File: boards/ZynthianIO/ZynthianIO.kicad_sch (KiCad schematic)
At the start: 27 parts, among them J1 Btn-1, J1 Raspberry_Pi_2_3, J10 Ctrl-2, J11 Display, J3 Btn-2, J7 Ctrl-3, J8 Ctrl-4, J9 Ctrl-1, U1 MCP23017_SP, U2 6N138, U3 74LS14

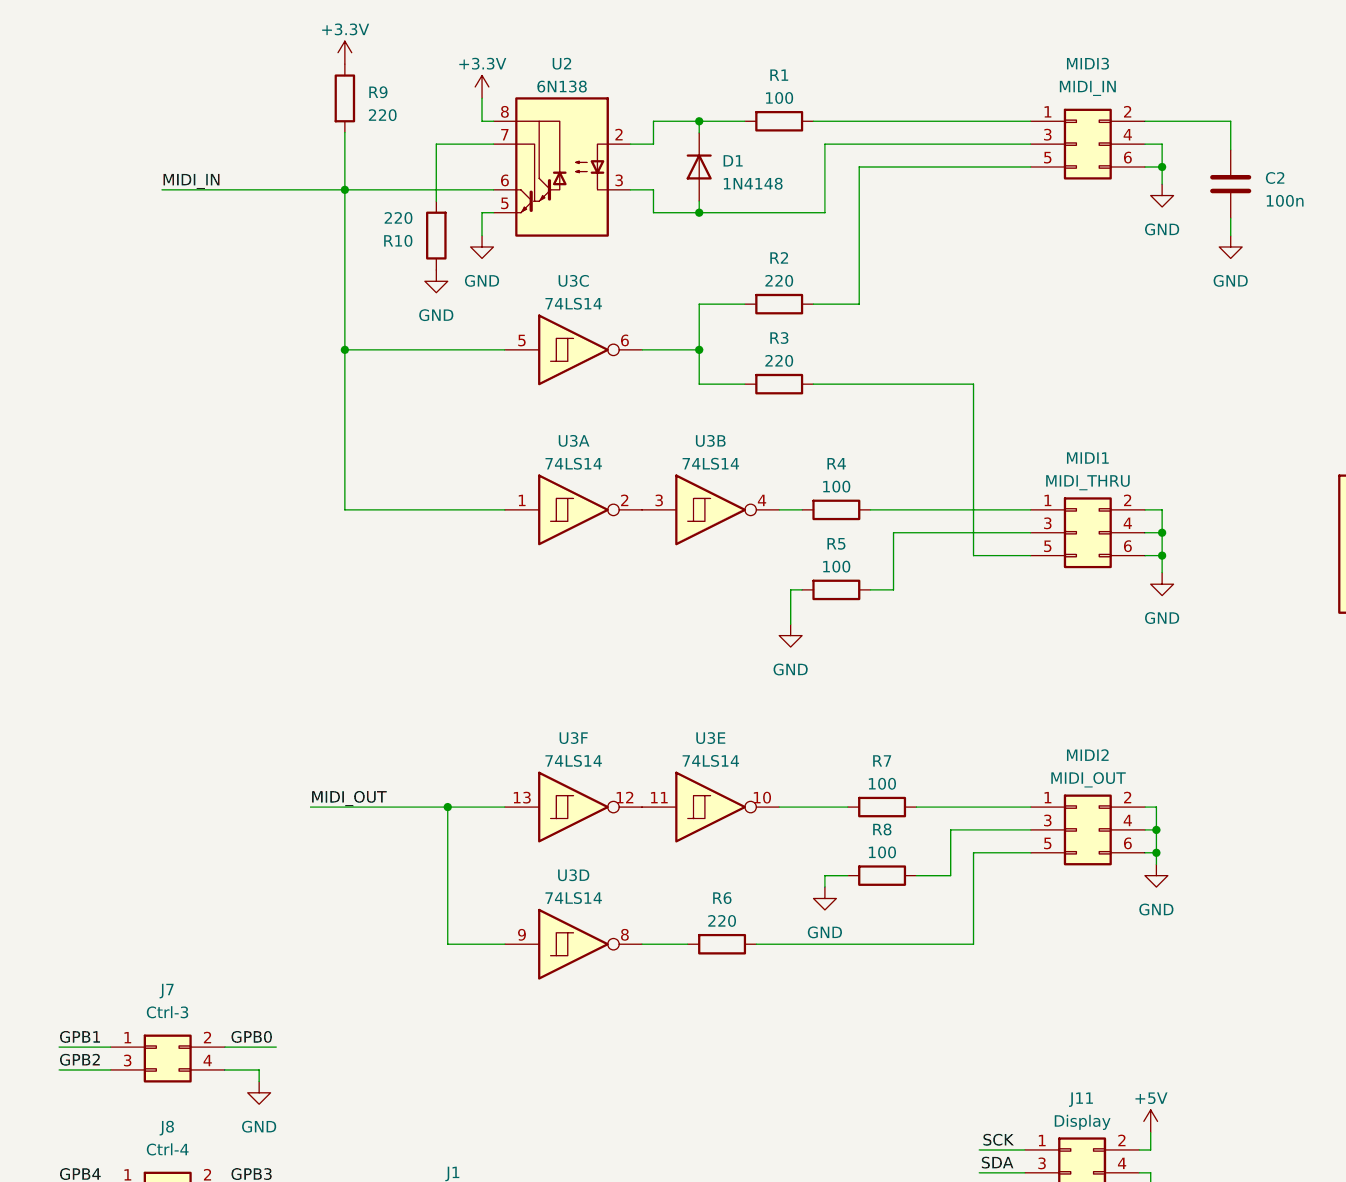
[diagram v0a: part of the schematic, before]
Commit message: Fixed MIDI interfaces
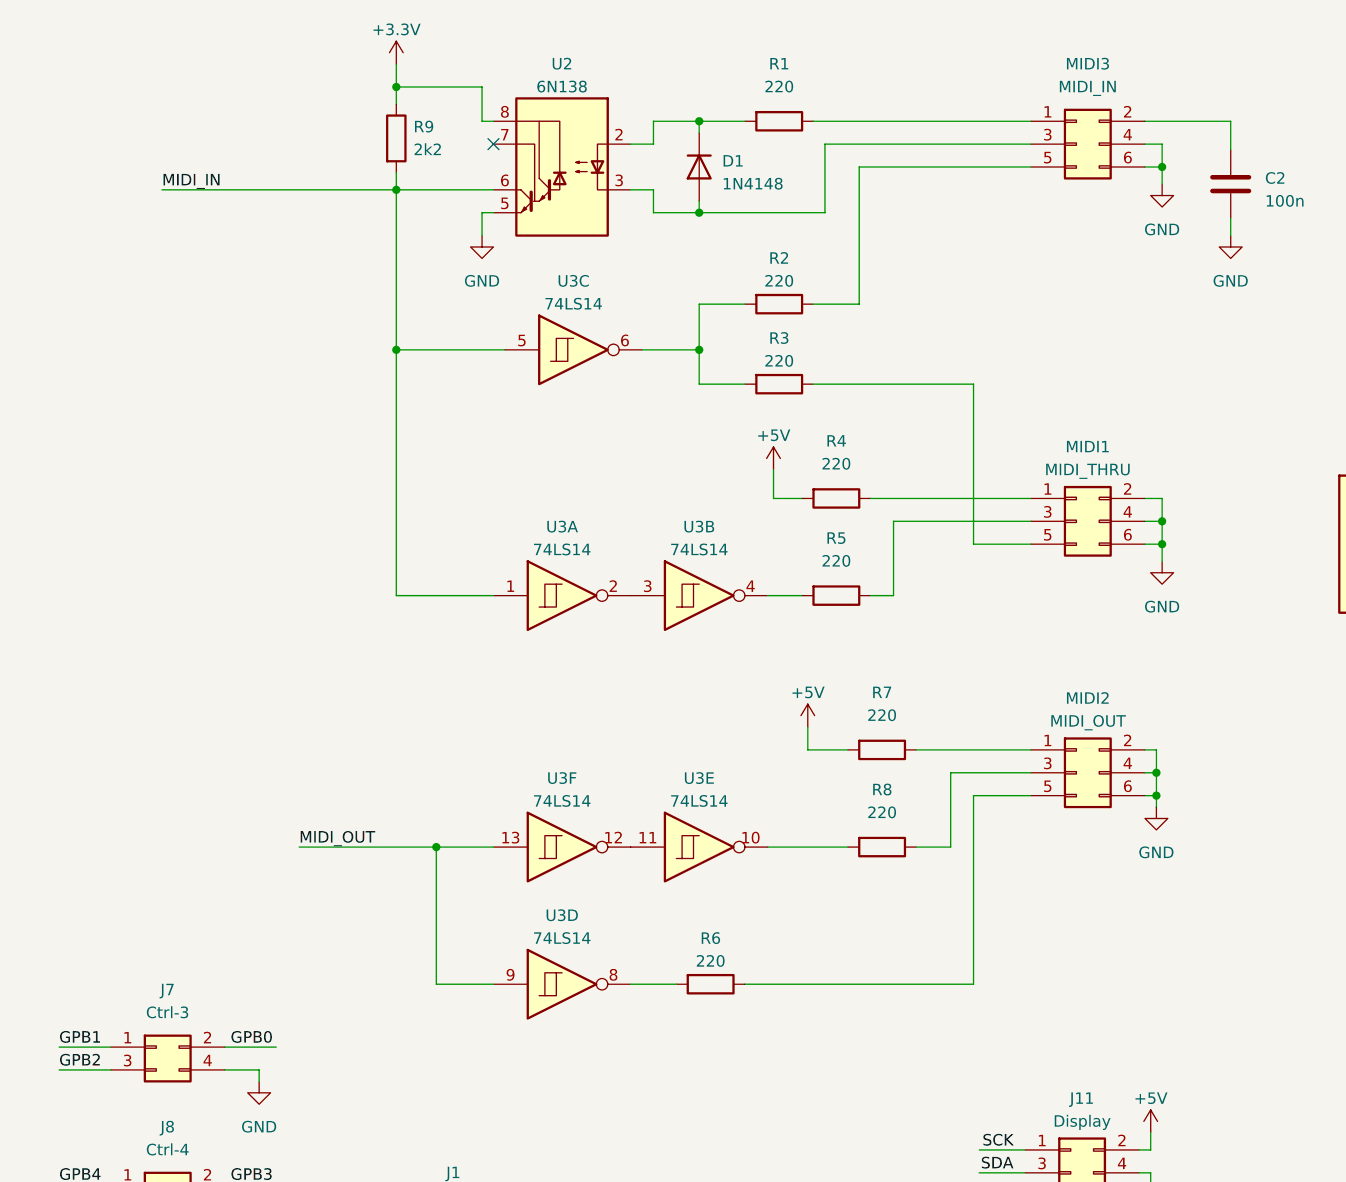
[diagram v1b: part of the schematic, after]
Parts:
- removed R10: 220, Resistor_THT:R_Axial_DIN0207_L6.3mm_D2.5mm_P7.62mm_Horizontal, symbol Device:R
- D1: footprint Diode_THT:D_DO-34_SOD68_P7.62mm_Horizontal -> Diode_THT:D_DO-35_SOD27_P7.62mm_Horizontal
- R1, R4, R5, R7, R8: value 100 -> 220
- R9: value 220 -> 2k2
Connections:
- net +5V: now also R4.2, R7.2
- net GND: no longer R5.2, R8.2
- net at U3.4: now also R5.2; no longer R4.2
- net at U3.10: now also R8.2; no longer R7.2
- no-connect marks 27 -> 28
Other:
- moved on the sheet: MIDI1, MIDI2, R4, R5, R6, R7, R8, R9, U3A, U3B, U3D, U3E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
